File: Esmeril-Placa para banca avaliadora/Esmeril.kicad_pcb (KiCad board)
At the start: 2 copper layers, 108 x 85.1 mm, 27 parts, among them J1 Entrada 12V, J10 CONTATOR, J2 Display OLED 0,96, J3 MFRC522, J4 MICRO SERVO 9G, J9 BUZER, SW1 RESET, SW2 RESET, SW3 ACRILICO, SW4 INFRAVERMELHO, SW5 PIR, SW6 MAGNETICO, U1 L7805, U2 L7803, U3 MOC3020M, U4 ESP-12E, U5 ATmega328P-PU, Y1 Crystal

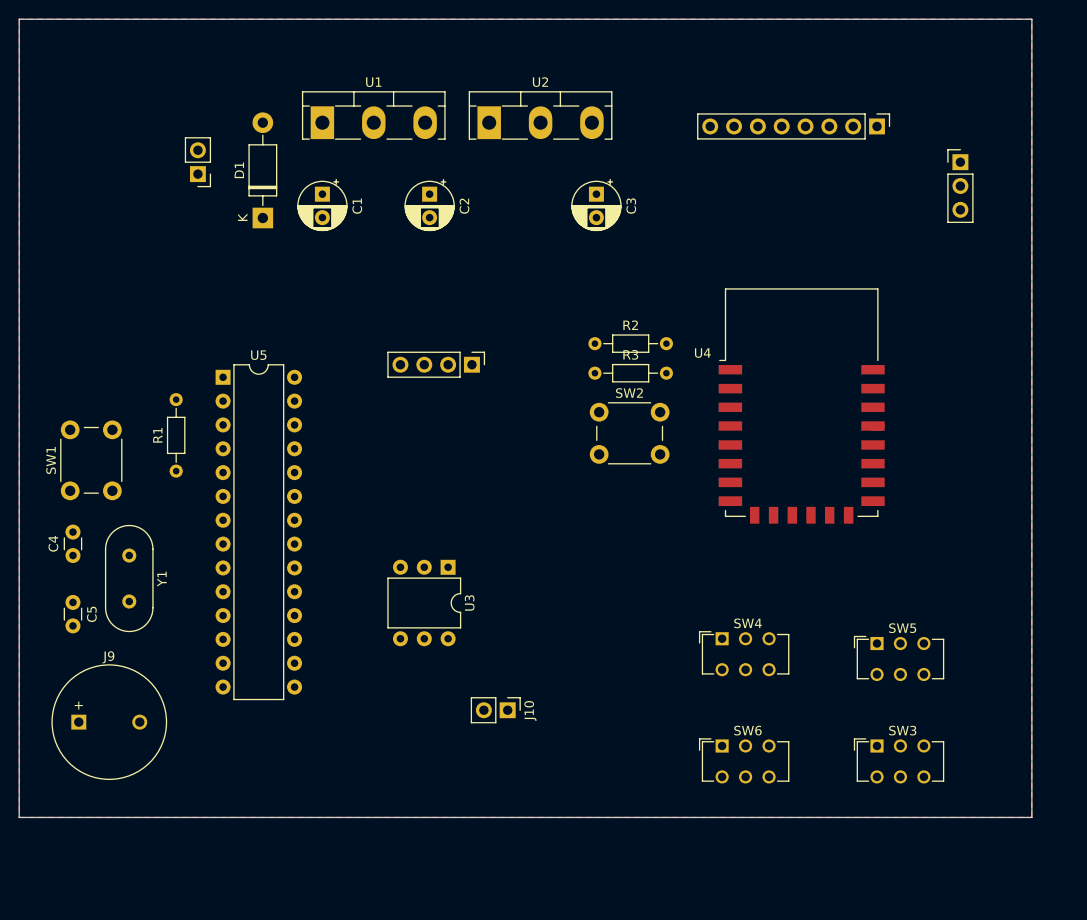
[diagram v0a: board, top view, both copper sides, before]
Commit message: Atualização
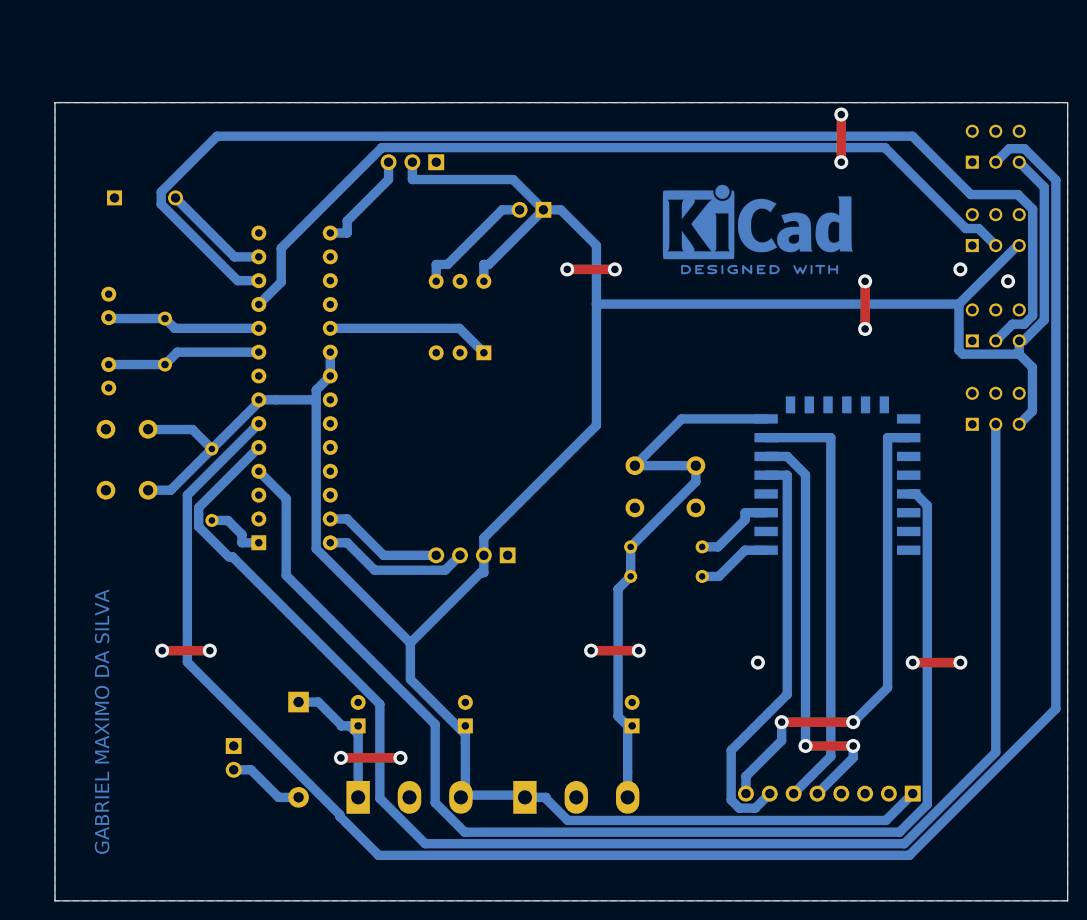
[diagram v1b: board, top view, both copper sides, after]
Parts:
- added REF**: KiCad-Logo2_8mm_B.CU, Symbol:KiCad-Logo2_8mm_B.CU, F.Cu at (180.3, 76.2)
- C1, C2, C3, C4, C5, D1, J1, J10, J2, J3, J4, J9, R1, R2, R3, SW1, SW2, SW3, SW4, SW5, SW6, U1, U2, U3, U4, U5, Y1: moved to B.Cu
- moved U1 72.0 mm to (137.7, 137.6)
- moved U2 72.0 mm to (155.5, 137.6)
- moved J3 71.2 mm to (196.8, 137.2), turned to 90 degrees
- moved SW6 67.7 mm to (203.2, 69.8)
- moved J1 61.1 mm to (124.5, 132.1)
- moved C1 56.8 mm to (137.7, 129.9), turned to 90 degrees
- moved C2 56.8 mm to (149.2, 129.9), turned to 90 degrees
- moved C3 56.8 mm to (166.9, 129.9), turned to 90 degrees
- moved J9 56.0 mm to (111.8, 73.7)
- moved J4 55.9 mm to (146.1, 69.8), turned to 90 degrees
- moved J10 53.5 mm to (157.5, 74.9), turned to 90 degrees
- moved D1 51.7 mm to (131.4, 127.4), turned to 270 degrees
- moved SW5 43.6 mm to (203.2, 78.7)
- moved SW4 41.5 mm to (203.2, 88.9)
- moved SW3 35.8 mm to (203.2, 97.8)
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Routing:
- net 5V: track 1.56 -> 312.3 mm
- net MAGNETICO: track 0.00 -> 201.0 mm
- net Acrilico: track 0.00 -> 154.9 mm
- net CARTAO: track 0.75 -> 132.5 mm
- net INFRAVERMELHO: track 0.00 -> 130.1 mm
- net PIR: track 0.00 -> 91.9 mm
- net 3,3V: track 0.00 -> 62.3 mm
- net SS: track 0.00 -> 50.9 mm, vias 0 -> 2
- net MOSI: track 0.00 -> 46.5 mm
- net MISO: track 0.00 -> 45.7 mm, vias 0 -> 2
- net SCK: track 0.00 -> 44.5 mm
- net GND: track 0.00 -> 36.8 mm, vias 0 -> 17
- net CONTATOR: track 0.00 -> 17.5 mm
- net CRISTAL1: track 0.00 -> 16.5 mm
- net CRISTAL2: track 0.14 -> 16.5 mm
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- added copper zone on B.Cu, net GND
- removed copper zone on F.Cu, net GND
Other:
- board text added: "GABRIEL MAXIMO DA SILVA"
